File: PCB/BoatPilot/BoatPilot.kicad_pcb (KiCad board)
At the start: 2 copper layers, 40 x 40 mm, 87 parts, among them J101 battery, J102 switch, J103 SWD, J104 wind, J105 RC, J106 GPS, J108 failsafe, J109 SERVO1, J110 SERVO2, J111 SERVO3, J201 GPIO, J202 USB-Audio-IR, J203 Audio-UART, P101 ICT-Point, P102 ICT-Point, P103 ICT-Point, P104 ICT-Point, P105 ICT-Point, P106 ICT-Point, P107 ICT-Point, P108 ICT-Point, P109 ICT-Point, P113 ICT-Point, P119 ICT-Point, P129 ICT-Point, P130 ICT-Point, P132 ICT-Point, P133 ICT-Point, P134 ICT-Point, P135 ICT-Point, Q101 TSM3457, U101 GY-91, U102 74LVC1G97, U103 LM1117-3.3, U104 TPS565208, U105 24LC512, U106 74LVC1G97, U108 74LVC1G97, U109 STM32F103C8Tx, Y101 8MHz

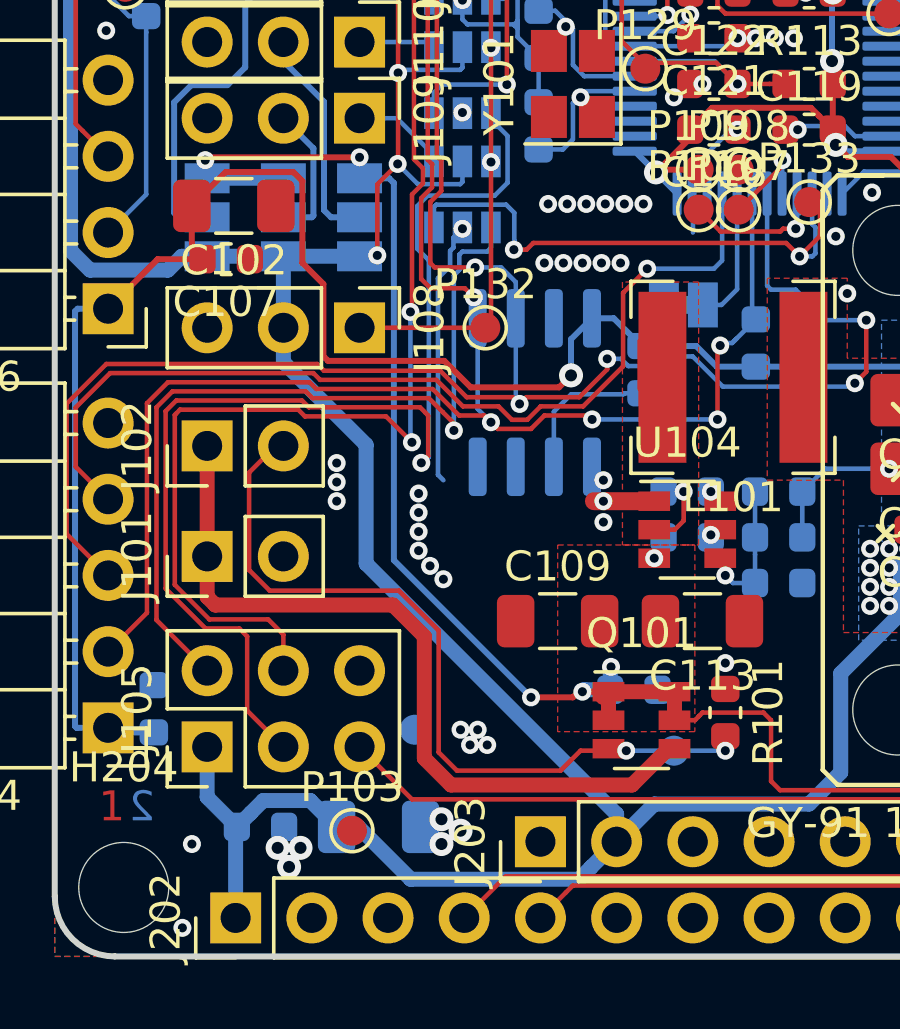
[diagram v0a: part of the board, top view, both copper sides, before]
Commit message: Add DMC to project
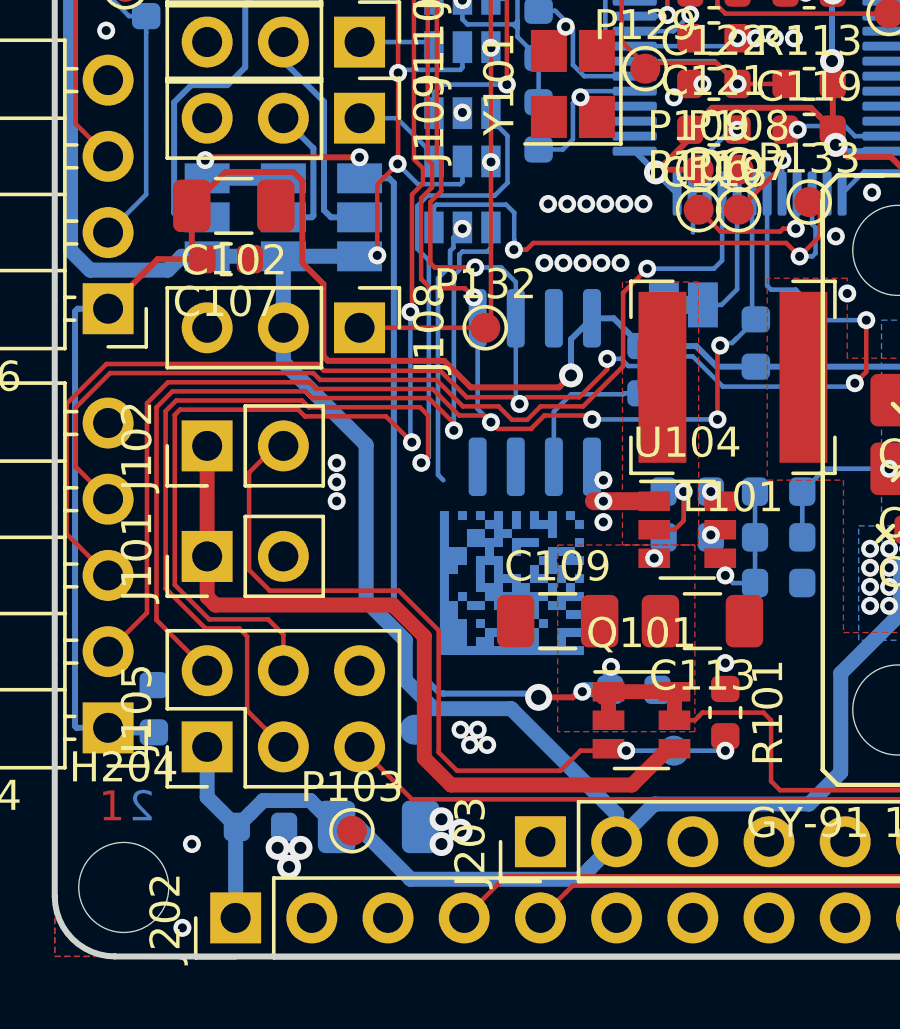
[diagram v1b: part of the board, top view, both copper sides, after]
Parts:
- added Barcode**: BoatPilot, footprint:BoatPilot, B.Cu at (139.2, 106.6)
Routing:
- net +BATT: track 53.1 -> 55.0 mm
- net +5V: track 115.5 -> 117.0 mm
- net GND: vias 75 -> 69
